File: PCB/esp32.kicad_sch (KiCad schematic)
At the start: 12 parts, among them SW1 RotaryEncoder_Switch, SW2 SW_Push, SW3 SW_Push, SW4 SW_Push, U7 ESP32-S3-WROOM-1

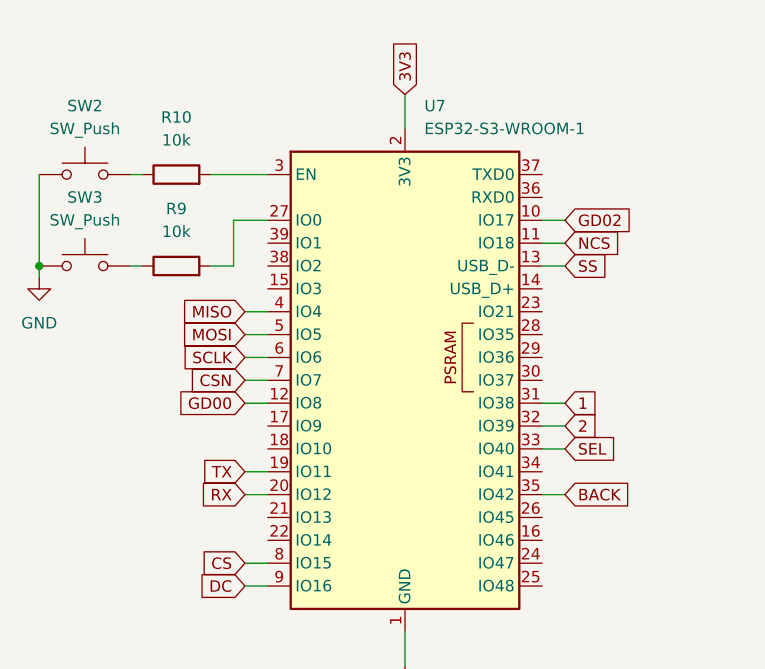
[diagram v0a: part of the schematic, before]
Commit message: Add files via upload
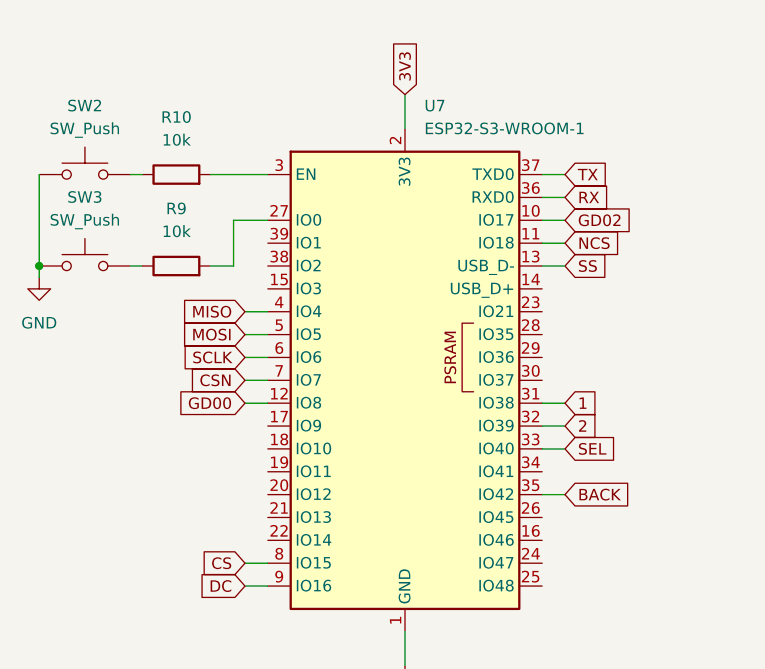
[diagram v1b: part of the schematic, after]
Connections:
- net RX: now also U7.36 (RXD0); no longer U7.20 (IO12)
- net TX: now also U7.37 (TXD0); no longer U7.19 (IO11)
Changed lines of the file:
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@@
-	(wire
-		(pts
-			(xy 125.73 114.3) (xy 128.27 114.3)
-		)
-		(stroke
-			(width 0)
-			(type default)
-		)
-	)
 	(wire
 		(pts
@@
 	(wire
 		(pts
-			(xy 125.73 111.76) (xy 128.27 111.76)
-		)
-		(stroke
-			(width 0)
-			(type default)
-		)
-	)
-	(wire
-		(pts
 			(xy 140.97 40.64) (xy 140.97 46.99)
 		)
@@
 	(wire
 		(pts
+			(xy 158.75 81.28) (xy 161.29 81.28)
+		)
+		(stroke
+			(width 0)
+			(type default)
+		)
+	)
+	(wire
+		(pts
 			(xy 30.48 40.64) (xy 30.48 45.72)
 		)
@@
 		(pts
 			(xy 157.48 40.64) (xy 158.75 40.64)
+		)
+		(stroke
+			(width 0)
+			(type default)
+		)
+	)
+	(wire
+		(pts
+			(xy 158.75 78.74) (xy 161.29 78.74)
 		)
 		(stroke
@@
 	(global_label "TX"
 		(shape input)
-		(at 125.73 111.76 180)
+		(at 161.29 78.74 0)
 		(fields_autoplaced yes)
 		(effects
@@
 				(size 1.27 1.27)
 			)
-			(justify right)
+			(justify left)
 		)
 		(property "Intersheetrefs" "${INTERSHEET_REFS}"
-			(at 120.5677 111.76 0)
+			(at 166.4523 78.74 0)
 			(hide yes)
 			(show_name no)
@@
 					(size 1.27 1.27)
 				)
-				(justify right)
+				(justify left)
 			)
 		)
@@
 	(global_label "RX"
 		(shape input)
-		(at 125.73 114.3 180)
+		(at 161.29 81.28 0)
 		(fields_autoplaced yes)
 		(effects
@@
 				(size 1.27 1.27)
 			)
-			(justify right)
+			(justify left)
 		)
 		(property "Intersheetrefs" "${INTERSHEET_REFS}"
-			(at 120.2653 114.3 0)
+			(at 166.7547 81.28 0)
 			(hide yes)
 			(show_name no)
@@
 					(size 1.27 1.27)
 				)
-				(justify right)
-			)
-		)
+				(justify left)
+			)
+		)
